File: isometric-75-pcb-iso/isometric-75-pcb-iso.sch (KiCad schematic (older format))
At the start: 26 parts, among them J101 USB, J102 SPI, J103 Conn_01x06_Male, Q101 AO3400A, SW101 RST, SW102 BOOT, U101 XC6206P332MR, U102 STM32F072CBTx

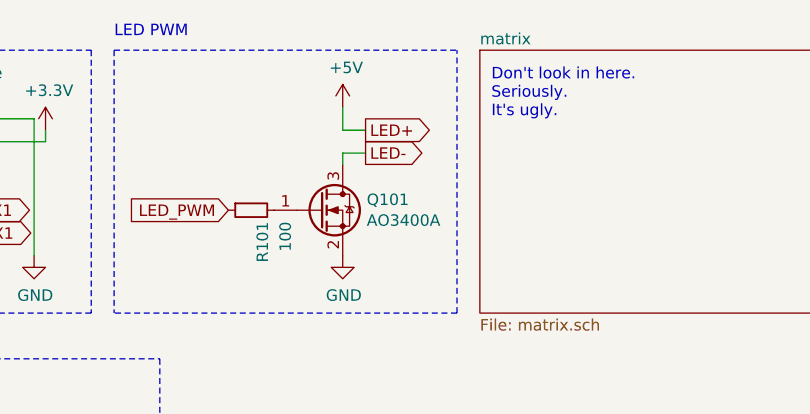
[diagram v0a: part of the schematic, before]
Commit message: minor layout fixes (thanks gLu3xb3rchi)
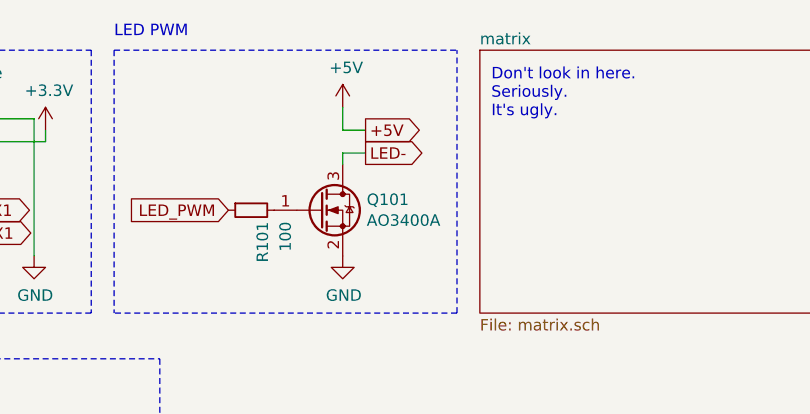
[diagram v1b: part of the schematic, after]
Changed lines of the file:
@@
 $EndComp
 Text GLabel 5700 1000 2    50   Output ~ 0
-LED+
++5V
 Text GLabel 5700 1100 2    50   Output ~ 0
 LED-
